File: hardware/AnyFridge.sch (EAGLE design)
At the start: 7 parts, among them U1 TSSP77038TT

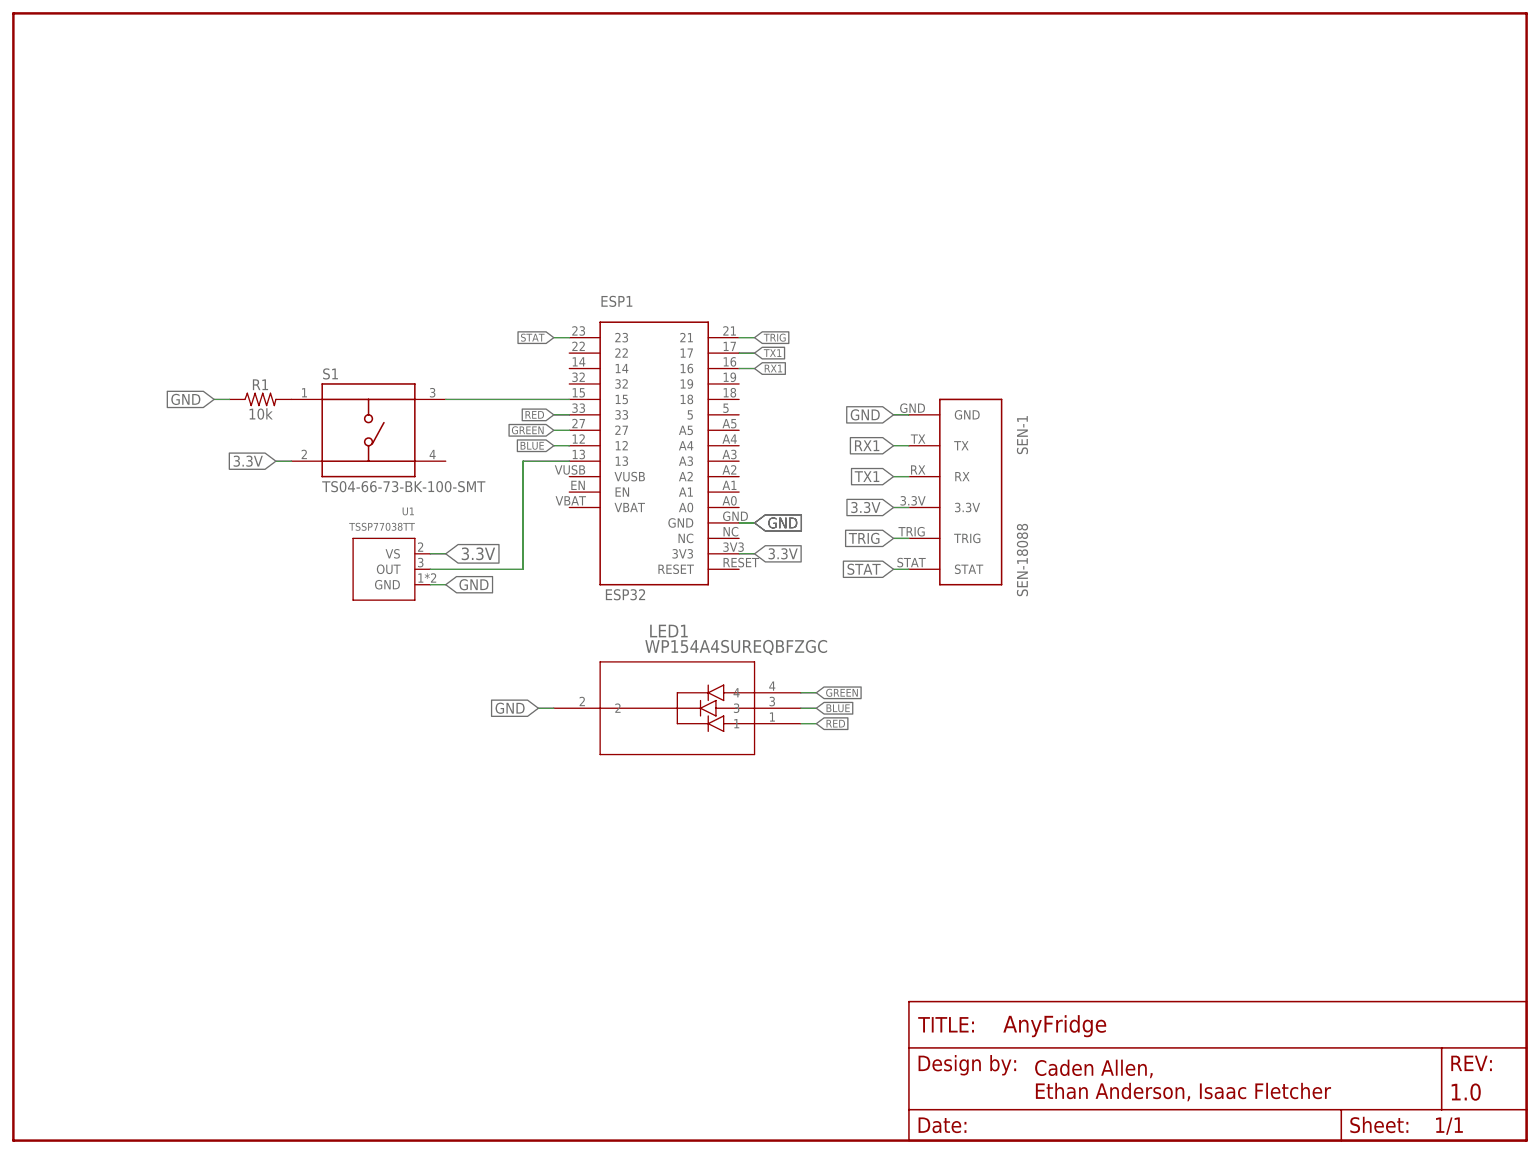
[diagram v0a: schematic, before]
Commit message: Updated schematic
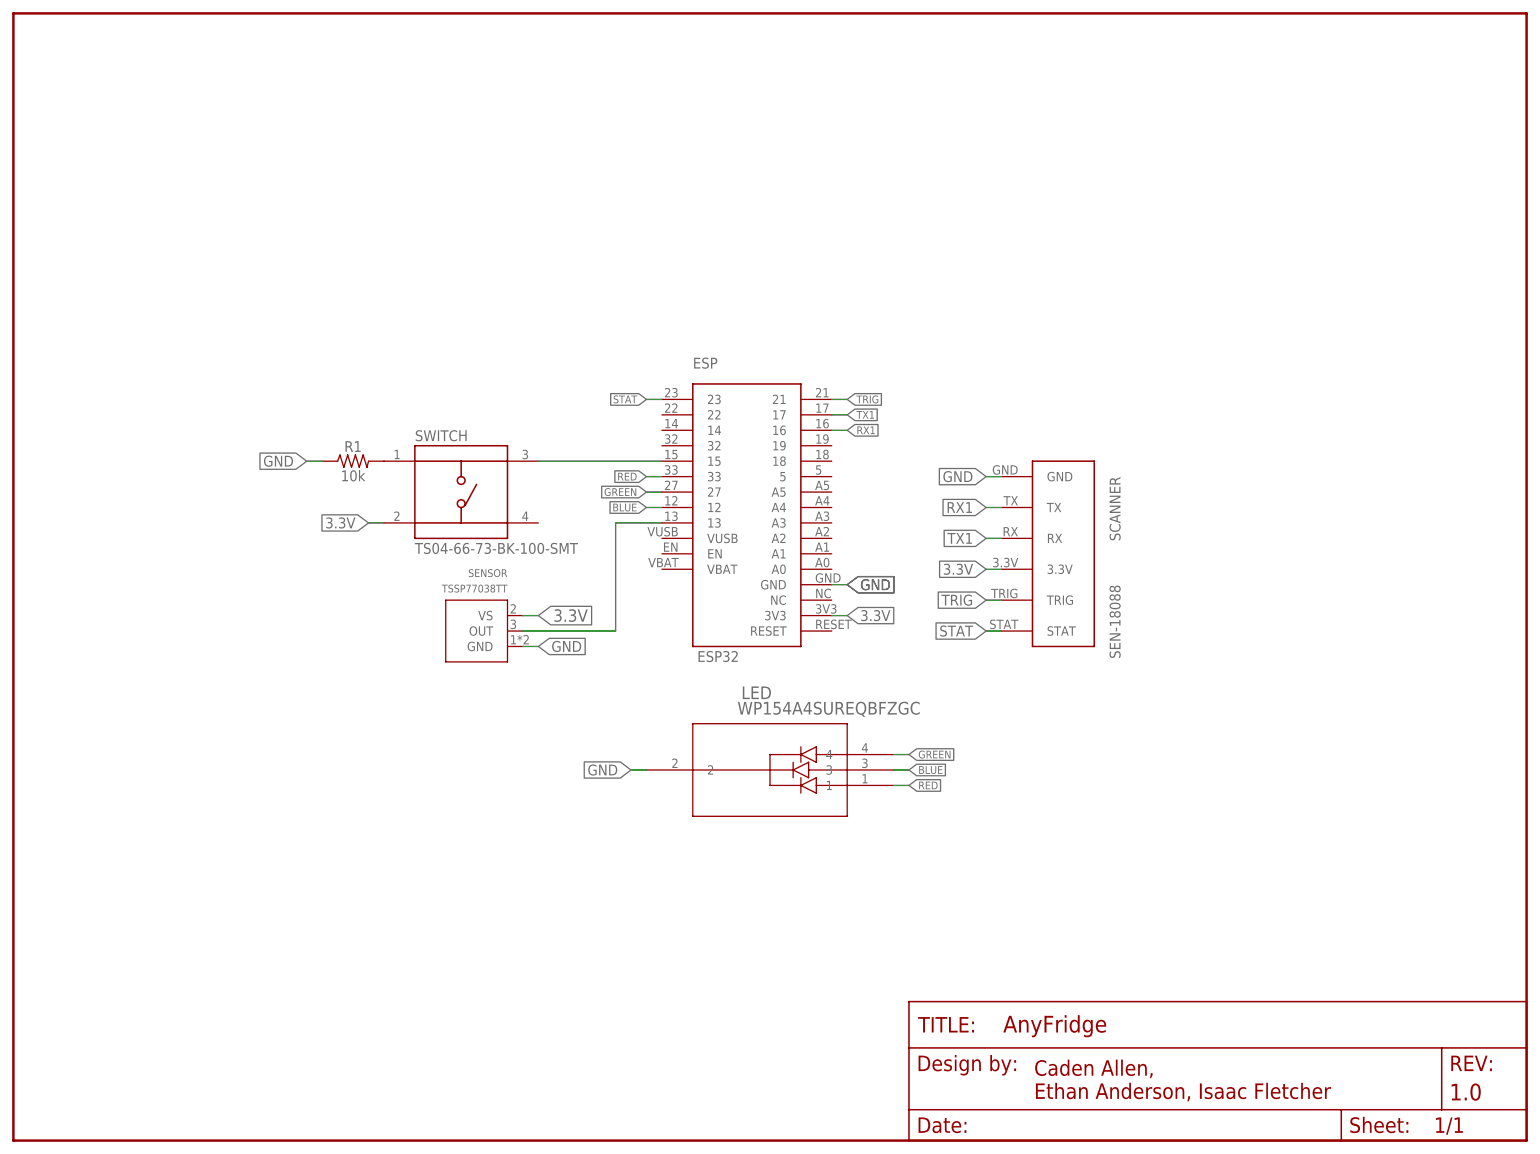
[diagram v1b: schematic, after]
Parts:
- removed ESP1: ESP32, ESP32:ESP32
- removed LED1: WP154A4SUREQBFZGC, MISC-PARTS:WP154A4SUREQBFZGC
- removed S1: TS04-66-73-BK-100-SMT, MISC-PARTS:TS04-66-73-BK-100-SMT
- removed SEN-1: SEN-18088, SEN-18088:SEN-18088
- removed U1: TSSP77038TT, MISC-PARTS:TSSP77038TT
- added ESP: ESP32, ESP32:ESP32
- added LED: WP154A4SUREQBFZGC, MISC-PARTS:WP154A4SUREQBFZGC
- added SCANNER: SEN-18088, SEN-18088:SEN-18088
- added SENSOR: TSSP77038TT, MISC-PARTS:TSSP77038TT
- added SWITCH: TS04-66-73-BK-100-SMT, MISC-PARTS:TS04-66-73-BK-100-SMT
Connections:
- net 3.3V: now also ESP.3V3, SCANNER.3.3V, SENSOR.VS, SWITCH.2; no longer ESP1.3V3, S1.2, SEN-1.3.3V, U1.VS
- net BLUE: now also ESP.12, LED.3; no longer ESP1.12, LED1.3
- net BUTTON: now also ESP.15, SWITCH.3; no longer ESP1.15, S1.3
- net GND: now also ESP.GND, LED.2, SCANNER.GND, SENSOR.GND; no longer ESP1.GND, LED1.2, SEN-1.GND, U1.GND
- net GREEN: now also ESP.27, LED.4; no longer ESP1.27, LED1.4
- net N$1: now also SWITCH.1; no longer S1.1
- net OUT: now also ESP.13, SENSOR.OUT; no longer ESP1.13, U1.OUT
- net RED: now also ESP.33, LED.1; no longer ESP1.33, LED1.1
- net RX1: now also ESP.16, SCANNER.TX; no longer ESP1.16, SEN-1.TX
- net STAT: now also ESP.23, SCANNER.STAT; no longer ESP1.23, SEN-1.STAT
- net TRIG: now also ESP.21, SCANNER.TRIG; no longer ESP1.21, SEN-1.TRIG
- net TX1: now also ESP.17, SCANNER.RX; no longer ESP1.17, SEN-1.RX
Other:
- moved on the sheet: R1
